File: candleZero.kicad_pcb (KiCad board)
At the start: 2 copper layers, 15 x 16 mm, 25 parts, among them J1 TEST_1P, J2 TEST_1P, J3 TEST_1P, J4 TEST_1P, J5 CONN_02X05, J6 DB9_MALE, U1 STM32F072C8Ux, U2 TLV70233DBV, U3 TJA1051TK/3

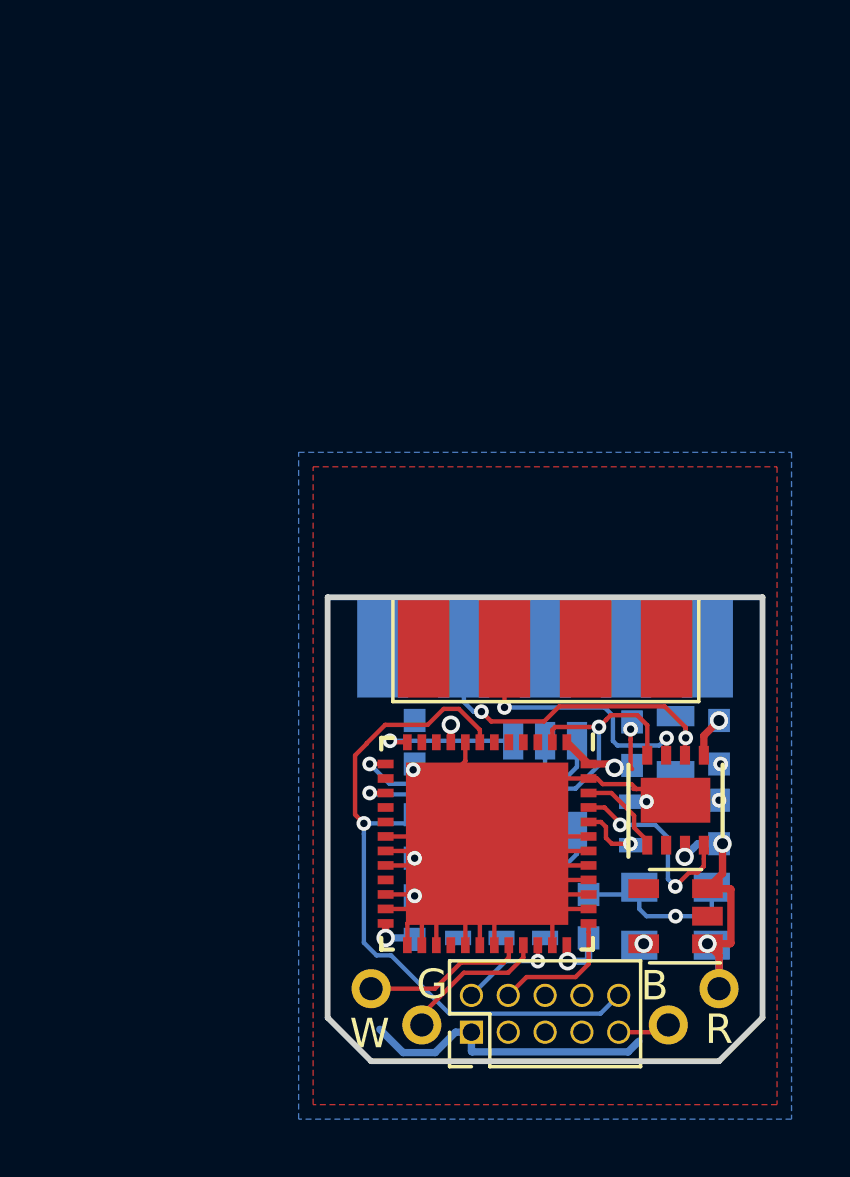
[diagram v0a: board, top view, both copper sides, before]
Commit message: v0.5 / bga design test
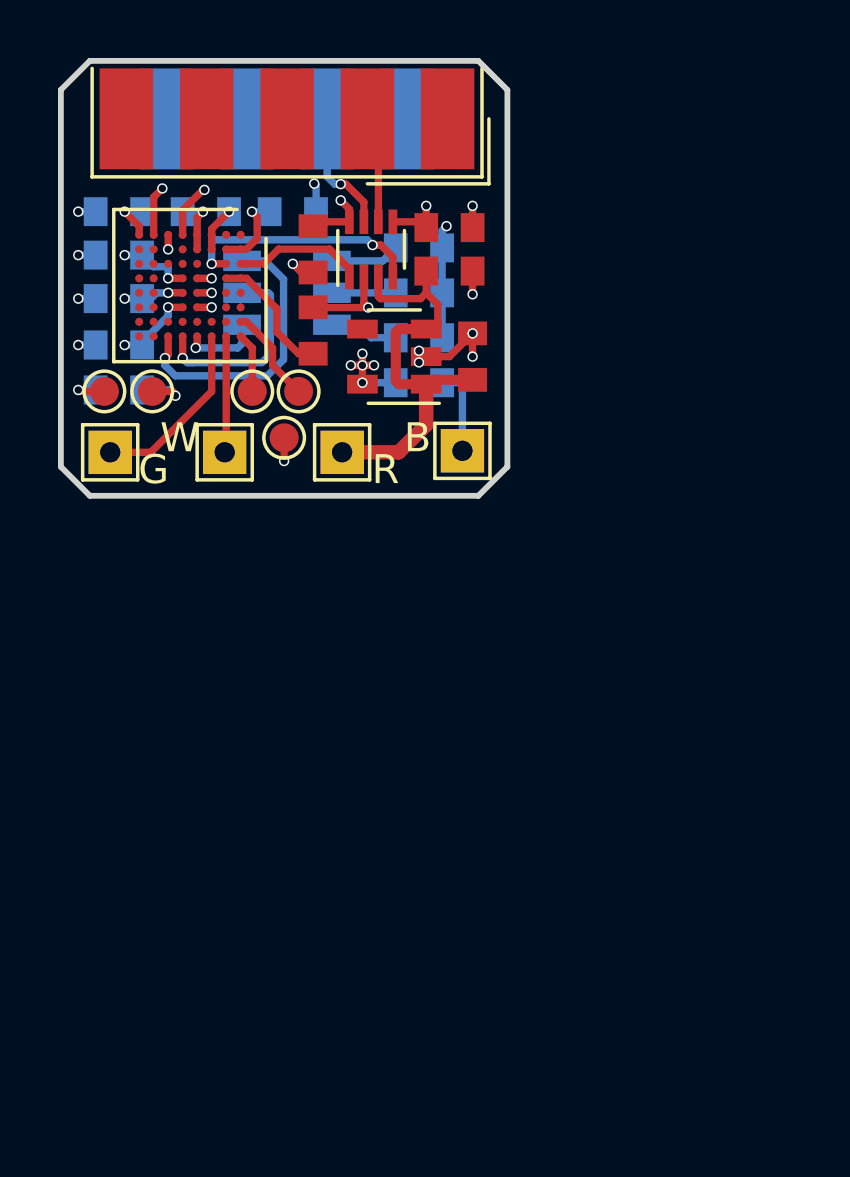
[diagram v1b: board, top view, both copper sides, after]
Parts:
- removed J2, J3, J4: TEST_1P, pins:Pin_Header_Straight_1x01_Pitch2.00mm
- removed J5: CONN_02X05, jtag:Pin_Header_Straight_2x05_Pitch1.27mm
- removed J6: DB9_MALE, subd9-small:DB9M_CI_SMALL
- removed R4: dnp, Resistors_SMD:R_0805
- removed R7: 120R, Resistors_SMD:R_0603
- added C10: 100nF, Capacitor_SMD:C_0603_1608Metric, B.Cu at (148.8, 73.2)
- added C11: 1uF, Capacitor_SMD:C_0603_1608Metric, B.Cu at (153.2, 79.1)
- added R1: R, Resistor_SMD:R_0603_1608Metric, B.Cu at (153.2, 74.5)
- added TP1: D-, TestPoint:TestPoint_THTPad_1.5x1.5mm_Drill0.7mm, F.Cu at (142.5, 81.5)
- added TP2: D+, TestPoint:TestPoint_THTPad_1.5x1.5mm_Drill0.7mm, F.Cu at (146.4, 81.5)
- added TP3: +5V, TestPoint:TestPoint_THTPad_1.5x1.5mm_Drill0.7mm, F.Cu at (150.5, 81.5)
- added TP4: GND, TestPoint:TestPoint_THTPad_1.5x1.5mm_Drill0.7mm, F.Cu at (154.7, 81.5)
- added TP5: VCC, TestPoint:TestPoint_Pad_D1.0mm, F.Cu at (148.5, 81.0)
- added TP6: RESET, TestPoint:TestPoint_Pad_D1.0mm, F.Cu at (143.9, 79.4)
- added TP7: SWDIO, TestPoint:TestPoint_Pad_D1.0mm, F.Cu at (147.4, 79.4)
- added TP8: SWCLK, TestPoint:TestPoint_Pad_D1.0mm, F.Cu at (149.0, 79.4)
- added TP9: GND, TestPoint:TestPoint_Pad_D1.0mm, F.Cu at (142.3, 79.4)
- C1, C2, C3, C5, C6, C8: footprint Capacitors_SMD:C_0603 -> Capacitor_SMD:C_0603_1608Metric
- C4: value 10uF/10V -> 100nF; footprint Capacitors_SMD:C_0805 -> Capacitor_SMD:C_0603_1608Metric; moved to F.Cu
- C7: value 10uF -> 1uF; footprint Capacitors_SMD:C_0805 -> Capacitor_SMD:C_0603_1608Metric; moved to F.Cu
- C9: value 100nF -> 1uF; footprint Capacitors_SMD:C_0603 -> Capacitor_SMD:C_0603_1608Metric; moved to F.Cu
- D1: footprint LEDs:LED_RGB_PLCC-6 -> LED_SMD:LED_RGB_PLCC-6
- J1: value TEST_1P -> DB9_Male; footprint pins:Pin_Header_Straight_1x01_Pitch2.00mm -> Connector_Dsub:DSUB-9_Male_EdgeMount_P2.77mm
- R2, R3: value 10K -> R; footprint Resistors_SMD:R_0603 -> Resistor_SMD:R_0603_1608Metric
- R5, R6: value 10R -> 10k; footprint Resistors_SMD:R_0603 -> Resistor_SMD:R_0603_1608Metric; moved to F.Cu
- U1: value STM32F072C8Ux -> STM32F072RBHx; footprint qfn48:QFN-48_EP_7x7_Pitch0.5mm -> Package_BGA:UFBGA-64_5x5mm_Layout8x8_P0.5mm
- U2: value TLV70233DBV -> TJA1051T-3; footprint TO_SOT_Packages_SMD:SOT-23-5 -> Package_DFN_QFN:DFN-8_2x2mm_P0.5mm
- U3: value TJA1051TK/3 -> TLV70233_SOT23-5; footprint Housings_DFN_QFN:DFN-8-1EP_3x3mm_Pitch0.65mm -> Package_TO_SOT_SMD:SOT-23-5
- moved J1 33.5 mm to (148.6, 70.0), turned to 180 degrees
- moved C6 29.5 mm to (142.8, 73.2), turned to 180 degrees
- moved C8 27.7 mm to (145.8, 73.2), turned to 0 degrees
- moved C4 25.4 mm to (154.2, 73.8), turned to 0 degrees
- moved U2 25.3 mm to (151.5, 74.5), turned to 90 degrees
- moved C5 24.8 mm to (142.8, 77.8), turned to 180 degrees
- moved R6 23.9 mm to (149.5, 74.5), turned to 270 degrees
- moved C3 23.7 mm to (142.8, 76.2), turned to 180 degrees
- moved C2 22.5 mm to (142.8, 74.7), turned to 180 degrees
- moved U1 21.8 mm to (145.2, 75.8)
- moved R5 20.8 mm to (149.5, 77.3)
- moved C7 20.1 mm to (155.0, 78.2)
- moved R2 19.7 mm to (153.2, 76.0), turned to 0 degrees
- moved D1 19.2 mm to (148.6, 76.0), turned to 0 degrees
- moved U3 18.1 mm to (152.3, 78.2), turned to 180 degrees
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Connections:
- C1 pad 1: +3V3 -> RESET
- C2 pad 1: NRST -> +3V3
- C4 pad 1: +5V -> +3V3
- C6 pad 1: +5V -> +3V3
- C7 pad 1: +3V3 -> +5V
- C9 pad 1: +3V3 -> GND
- C9 pad 2: GND -> +5V
- D1 pad 1: LED_B -> R
- D1 pad 2: LED_G -> G
- D1 pad 3: LED_R -> B
- J1 pad 1: +5V -> Net-(J1-Pad1)
- R2 pad 1: /BOOT -> Net-(D1-Pad5)
- R2 pad 2: GND -> +3V3
- R3 pad 1: +3V3 -> Net-(D1-Pad6)
- R3 pad 2: CAN_S -> +3V3
- R5 pad 1: +3V3 -> BOOT0
- R5 pad 2: Net-(D1-Pad6) -> GND
- R6 pad 1: +3V3 -> SILENT
- R6 pad 2: Net-(D1-Pad5) -> +3V3
- U2 pad 1: +5V -> TXD
- U2 pad 4: (no net) -> RXD
- U3 pad 1: CAN_TX -> +5V
- U3 pad 4: CAN_RX -> Net-(U3-Pad4)
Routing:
- net GND: track 66.0 -> 18.9 mm, vias 8 -> 18
- net NRST: track 24.1 -> 0.00 mm, vias 1 -> 0
- net RESET: track 0.00 -> 16.6 mm, vias 0 -> 2
- net CAN_S: track 12.3 -> 0.00 mm, vias 1 -> 0
- net /CAN_L: track 12.2 -> 0.00 mm, vias 2 -> 0
- net /CAN_H: track 10.7 -> 0.00 mm, vias 2 -> 0
- net SILENT: track 0.00 -> 10.6 mm, vias 0 -> 2
- net B: track 0.00 -> 9.98 mm, vias 0 -> 1
- net LED_R: track 9.01 -> 0.00 mm, vias 1 -> 0
- net RXD: track 0.00 -> 8.48 mm, vias 0 -> 2
- net LED_G: track 7.97 -> 0.00 mm, vias 1 -> 0
- net G: track 0.00 -> 7.15 mm, vias 0 -> 1
- net CAN_RX: track 6.99 -> 0.00 mm, vias 2 -> 0
- net +3V3: track 18.2 -> 24.5 mm, vias 6 -> 18
- net D-: track 0.00 -> 6.27 mm
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- added copper zone on In1.Cu, net +3V3
- added copper zone on In2.Cu, net GND
- removed copper zone on B.Cu, net +3V3
- removed copper zone on F.Cu, net GND
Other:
- board size 15 x 16 mm -> 15.4 x 15 mm
- copper layers 2 -> 4
- net class 3V3 removed
- net class 5V removed
- net class CAN removed
- net class Default: clearance 0.1524 -> 0.2; trace_width 0.1524 -> 0.254; via_dia 0.508 -> 0.36
- rule pad_to_mask_clearance: 0.0254 -> 0.0508
- rule trace_clearance: 0.1524 -> 0.2
- rule trace_min: 0.1524 -> 0.127
- rule via_min_size: 0.508 -> 0.36
- board text added: "Zero"
- board text added: "candle"
- board text added: "v0.5"
- board text removed: "candleZero"
- board text removed: "v0.4"
